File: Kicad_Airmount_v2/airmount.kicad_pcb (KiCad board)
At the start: 2 copper layers, 24.1 x 28.1 mm, 4 parts, among them J1 JST, M1 Motor_DC, M2 Motor_DC

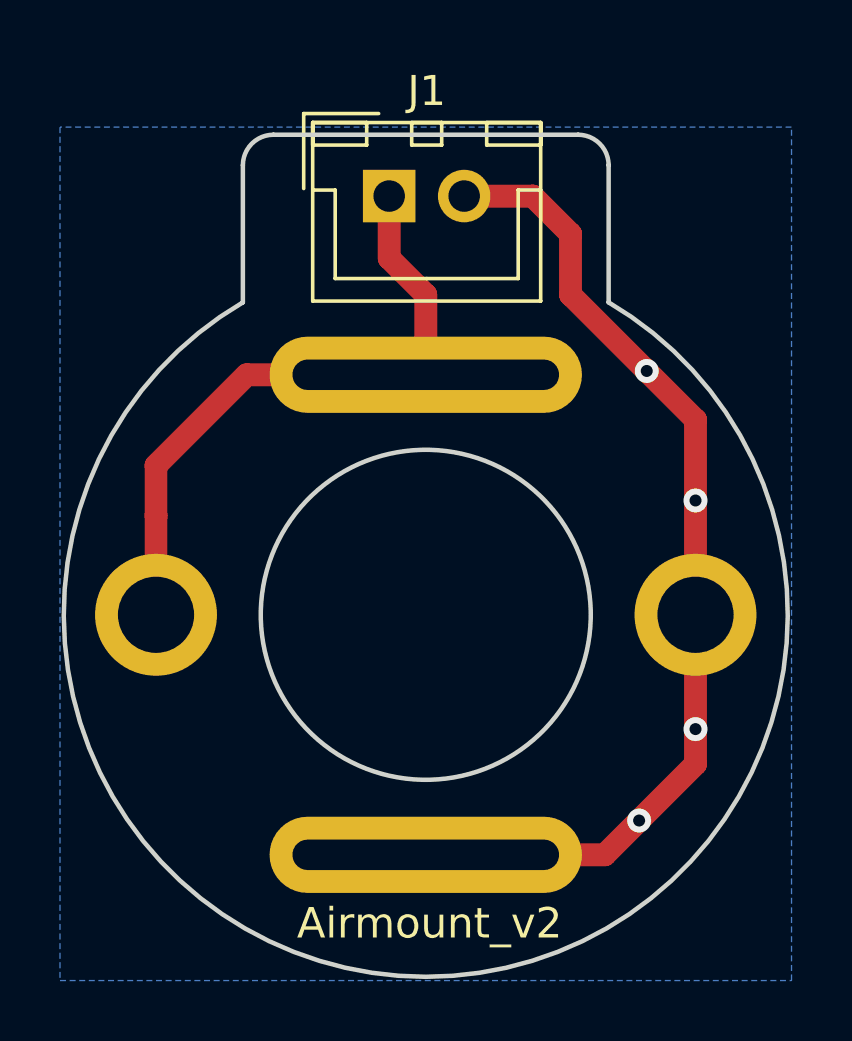
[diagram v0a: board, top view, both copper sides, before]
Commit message: Airmount _v2 and _v3 revised gerbers
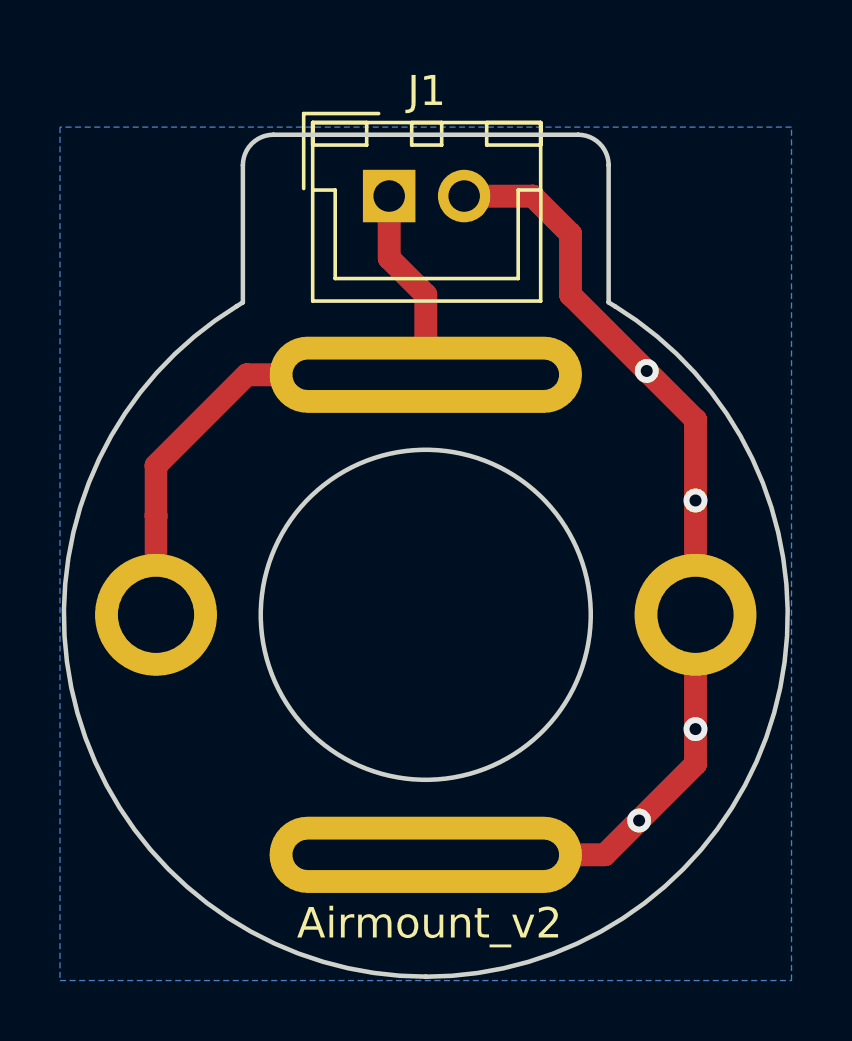
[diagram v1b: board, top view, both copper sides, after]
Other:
- outline, holes or cut-outs redrawn
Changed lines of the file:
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@@
   (general
     (thickness 1.6)
-    (drawings 11)
+    (drawings 14)
     (tracks 23)
     (zones 0)
@@
     (47 F.CrtYd user)
     (48 B.Fab user)
-    (49 F.Fab user)
+    (49 F.Fab user hide)
   )
   (setup
@@
     )
   )
+  (gr_line (start 120.7008 78.613) (end 120.904 78.486) (layer Edge.Cuts) (width 0.15))
+  (gr_arc (start 127 88.9) (end 120.700801 78.613001) (angle -148.5189608) (layer Edge.Cuts) (width 0.15))
+  (gr_line (start 133.2992 78.613) (end 133.096 78.486) (layer Edge.Cuts) (width 0.15))
+  (gr_arc (start 127 88.9) (end 127 100.965) (angle -148.5189608) (layer Edge.Cuts) (width 0.15))
   (gr_text Airmount_v2 (at 127.127 99.187) (layer F.SilkS)
     (effects (font (size 1.016 1.016) (thickness 0.1524)))
@@
   (gr_line (start 133.096 78.486) (end 133.096 73.914) (layer Edge.Cuts) (width 0.15))
   (gr_circle (center 127 88.9) (end 132.5 88.9) (layer Edge.Cuts) (width 0.15))
-  (gr_arc (start 127 88.9) (end 120.904 78.486) (angle -299.3135022) (layer Edge.Cuts) (width 0.15))
   (segment (start 132.969 96.901) (end 127 96.901) (width 0.762) (layer F.Cu) (net 1))
   (segment (start 135.9916 93.8784) (end 134.112 95.758) (width 0.762) (layer F.Cu) (net 1))
